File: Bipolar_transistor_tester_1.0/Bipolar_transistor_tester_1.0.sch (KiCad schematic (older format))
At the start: 0 parts

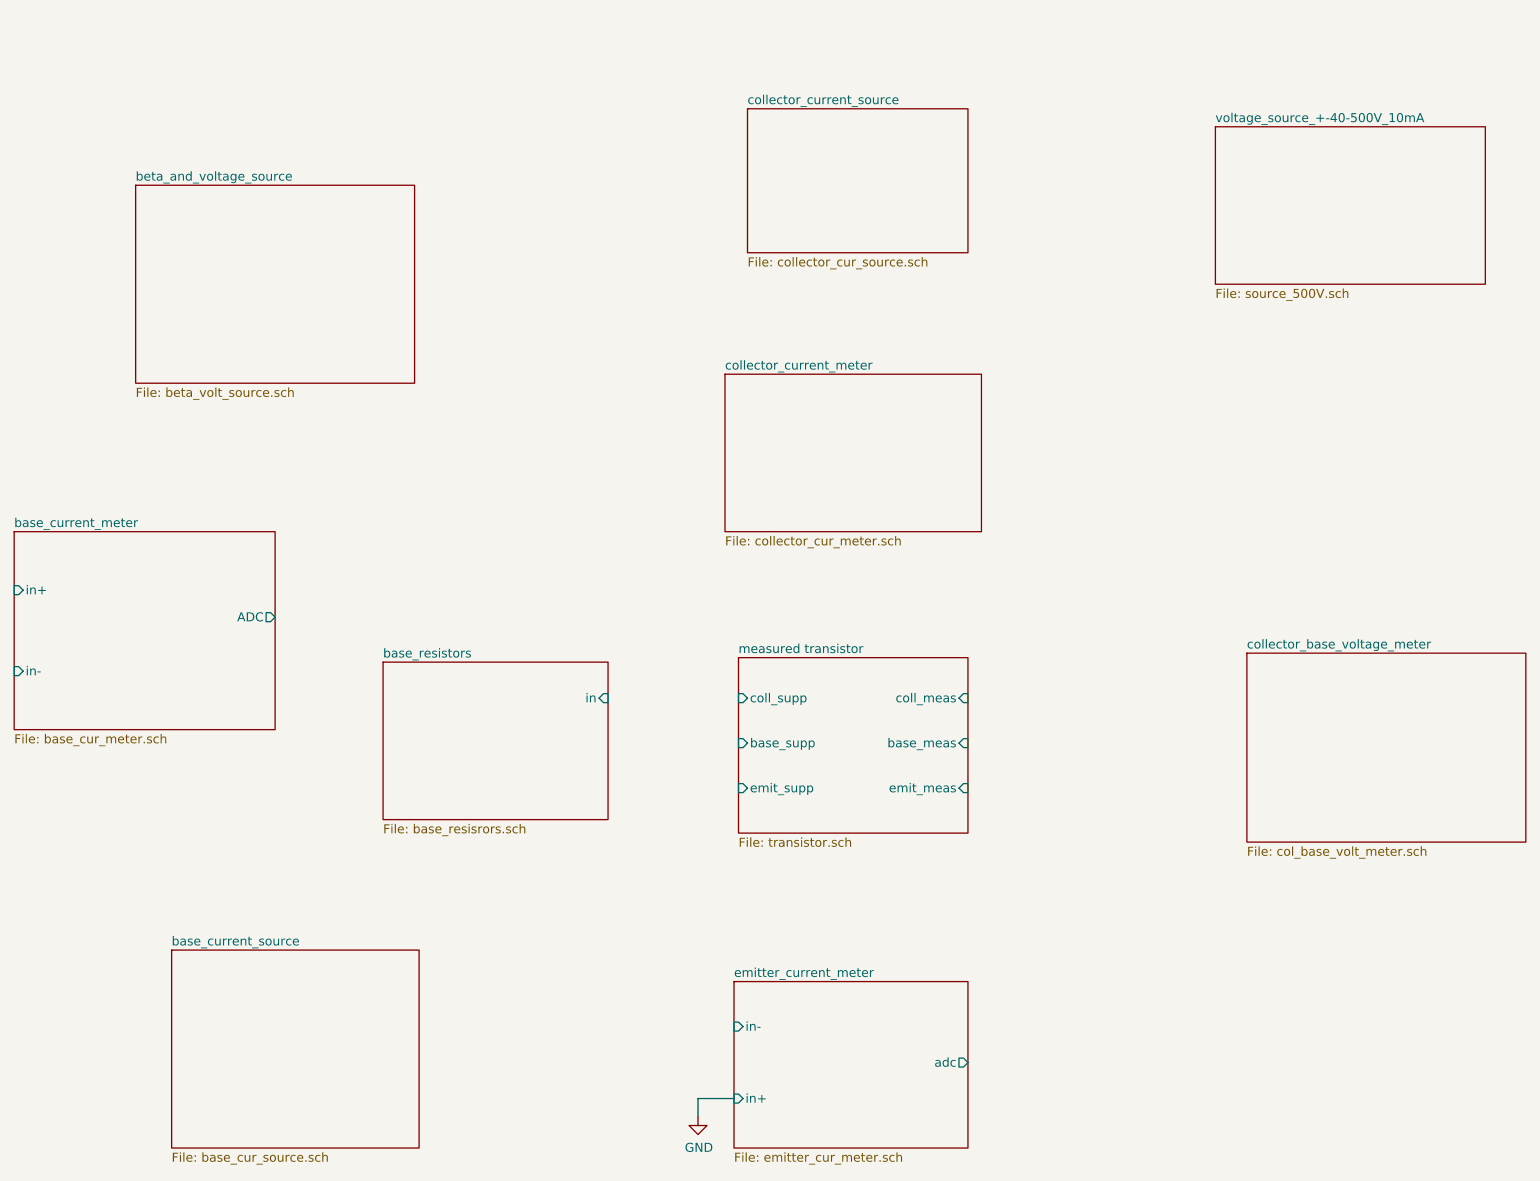
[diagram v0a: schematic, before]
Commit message: tester up
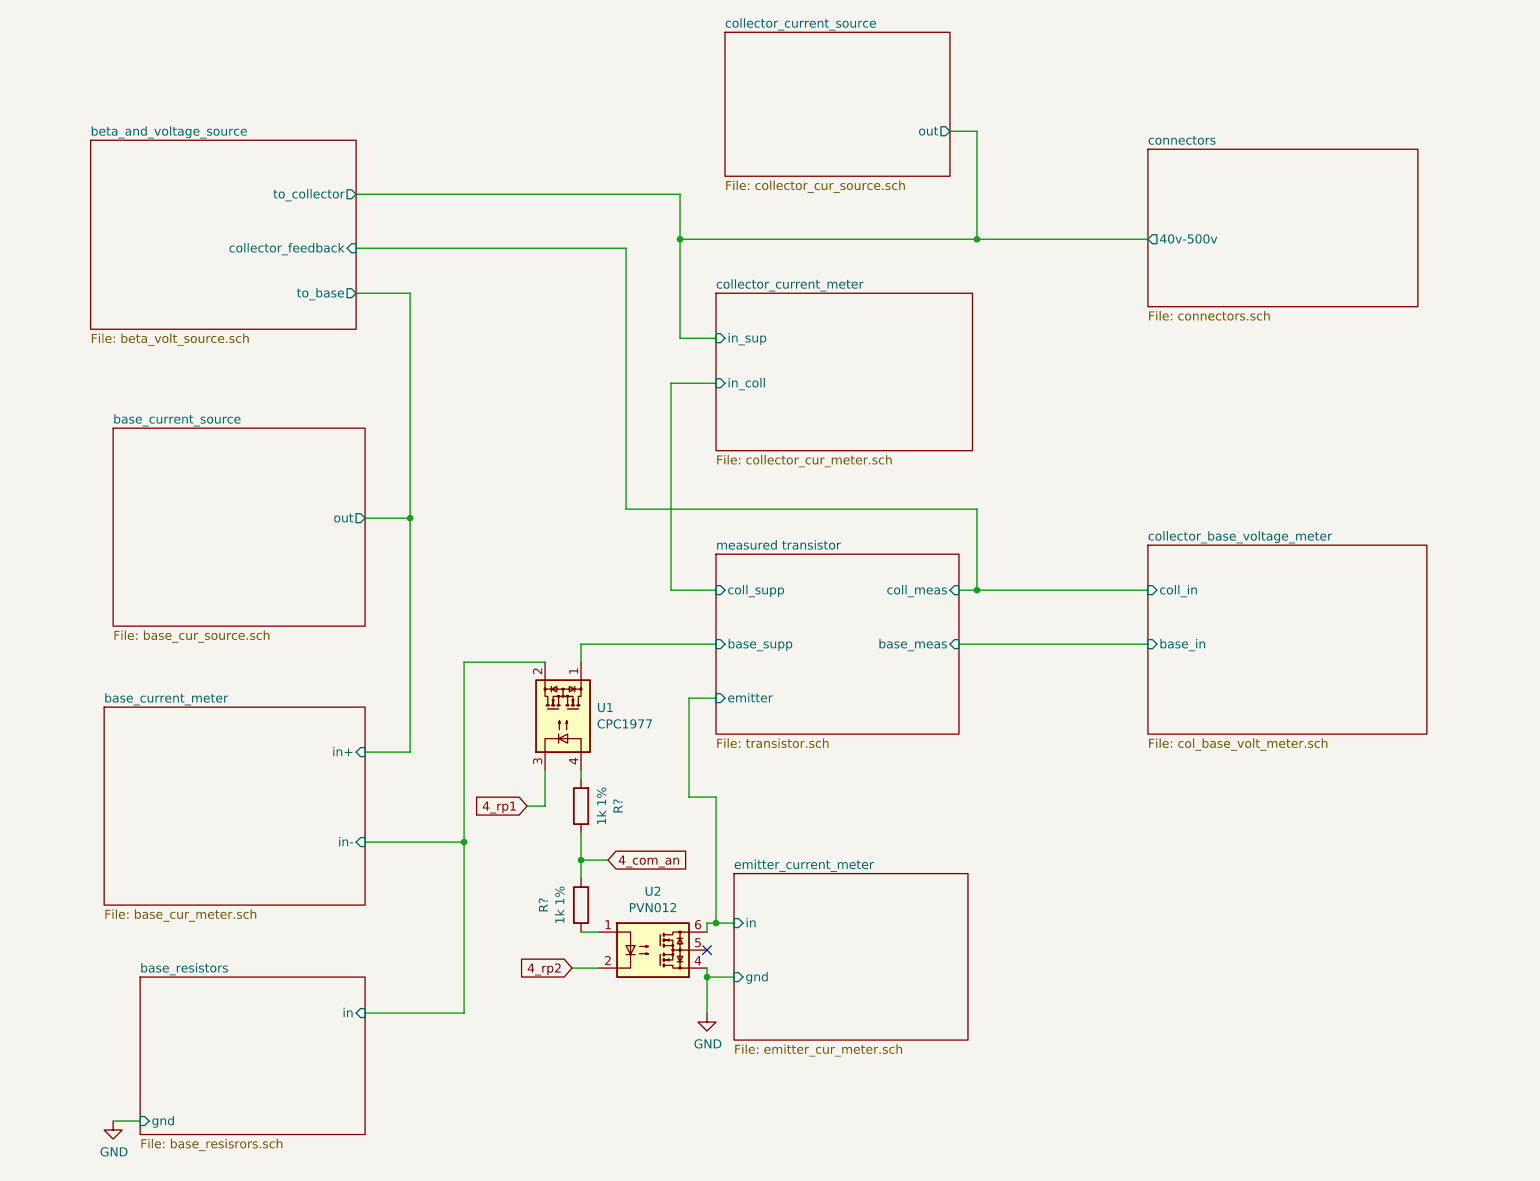
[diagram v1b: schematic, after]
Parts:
- added R? (x2): 1k 1%, Resistor_SMD:R_0805_2012Metric, symbol Device:R
- added U1: CPC1977, OptoDevice:i4-PAC, symbol Relay_SolidState:CPC1977
- added U2: PVN012, Package_DIP:DIP-6_W7.62mm, symbol Relay_SolidState:PVN012
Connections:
- net GND: now also U2.4
- net base_current_meter/in-: now also U1.2
- net measured transistor/base_supp: now also U1.1
- new net: R?.2, U2.1
- new net: R?.2, U1.4
- new net 4_com_an: R?.1, R?.1
- new net 4_rp1: U1.3
- new net 4_rp2: U2.2
- new net emitter_current_meter/in: U2.6
- no-connect marks 0 -> 1
